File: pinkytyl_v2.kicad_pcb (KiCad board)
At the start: 2 copper layers, 132.2 x 106 mm, 58 parts, among them J1 STX-3501-3N, J2 Conn_01x02, J3 USB_B_Mini, J5 Conn_02x05_Odd_Even, K0 KEYSW, K10 KEYSW, K11 KEYSW, K12 KEYSW, K13 KEYSW, K14 KEYSW, K15 KEYSW, K20 KEYSW, K21 KEYSW, K22 KEYSW, K23 KEYSW, K24 KEYSW, K25 KEYSW, K30 KEYSW, K31 KEYSW, K32 KEYSW, K33 KEYSW, K34 KEYSW, K35 KEYSW, K40 KEYSW, K41 KEYSW, U1 ATmega32U4-MU, Y1 Crystal_GND24_Small

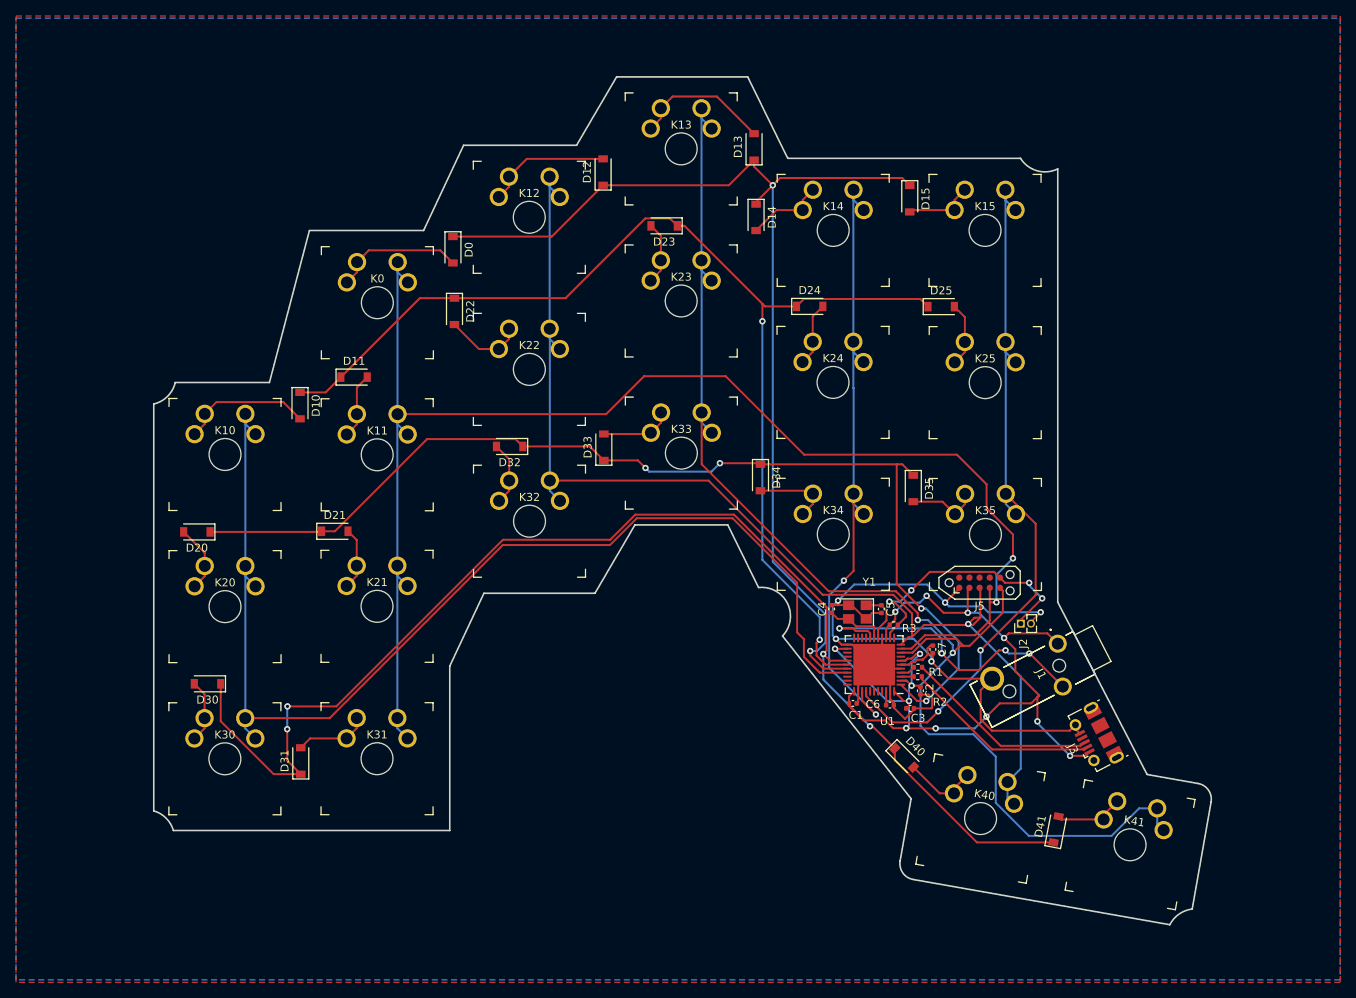
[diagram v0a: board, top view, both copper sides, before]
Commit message: In the middle of slim redesign
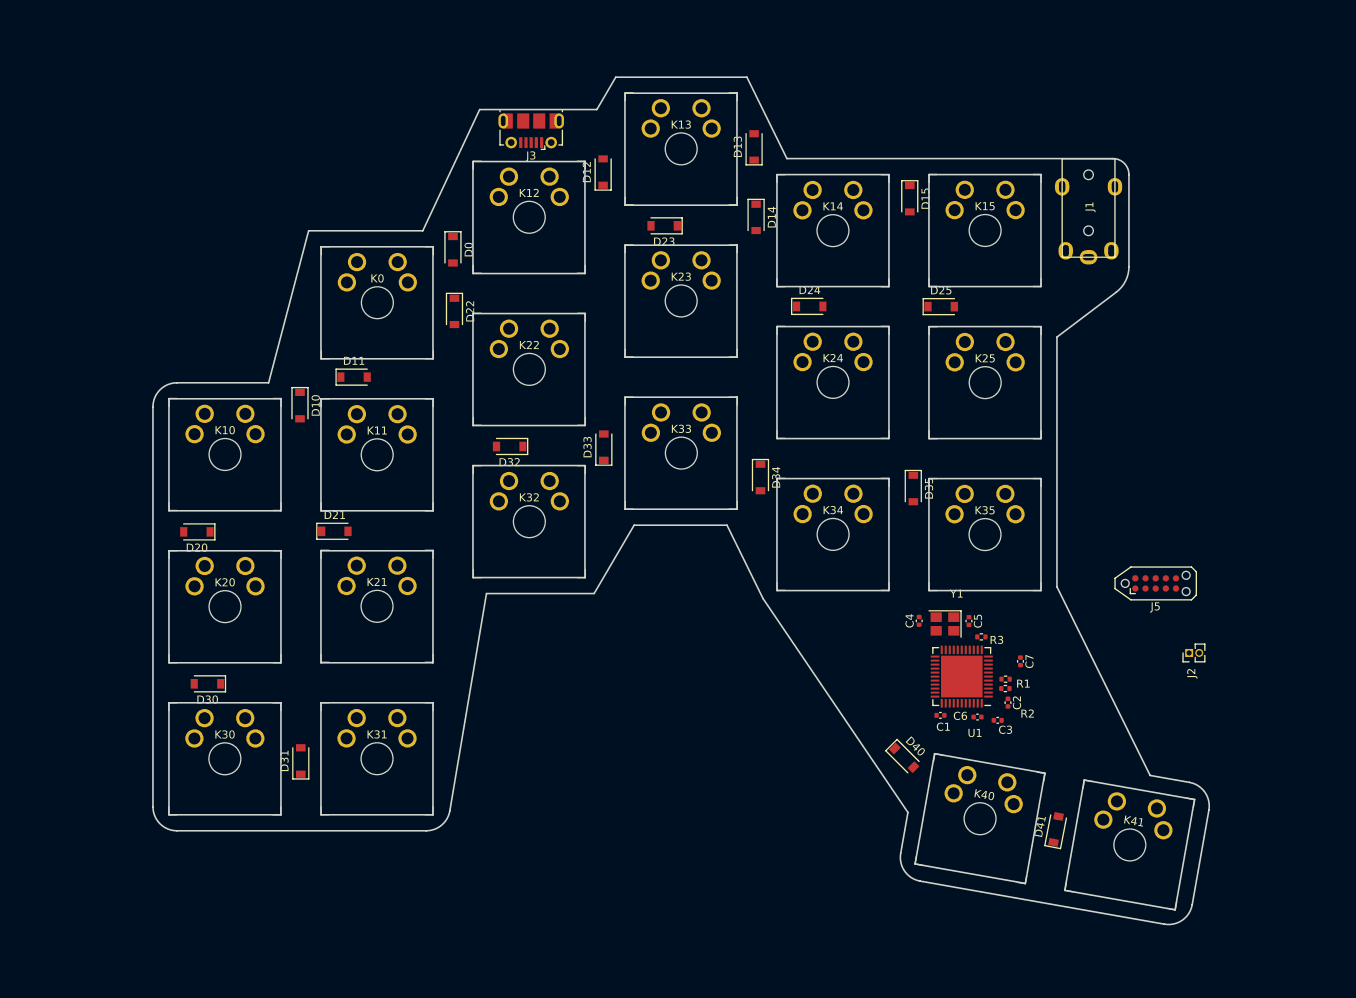
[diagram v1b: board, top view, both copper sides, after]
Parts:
- J1: value STX-3501-3N -> 50-00174; footprint STX-3501-3N:STX35013N -> misc:54-00174
- moved J3 103.5 mm to (117.8, 42.9), turned to 180 degrees
- moved J1 60.7 mm to (187.5, 46.4), turned to 270 degrees
- moved J5 22.0 mm to (195.9, 99.5)
- moved J2 21.4 mm to (200.1, 108.2)
- moved R1 11.1 mm to (177.2, 111.4)
- moved R2 11.1 mm to (177.1, 112.6)
- moved R3 11.1 mm to (174.1, 106.1)
- moved Y1 11.1 mm to (169.6, 104.5)
- moved C1 11.1 mm to (169.0, 116.0)
- moved C7 11.1 mm to (179.0, 109.2)
- moved C2 11.1 mm to (177.4, 114.4)
- moved C3 11.1 mm to (176.2, 116.6)
- moved C4 11.1 mm to (166.3, 104.1)
- moved C5 11.1 mm to (172.6, 104.2)
- moved C6 11.1 mm to (173.6, 116.2)
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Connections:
- J1 pad 2: GND -> serial
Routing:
- net MOSI: track 185.0 -> 0.00 mm, vias 2 -> 0
- net c3: track 171.3 -> 0.00 mm, vias 2 -> 0
- net r0: track 159.4 -> 0.00 mm, vias 4 -> 0
- net c0: track 145.8 -> 0.00 mm
- net MISO: track 144.7 -> 0.00 mm, vias 1 -> 0
- net r2: track 144.3 -> 0.00 mm, vias 2 -> 0
- net r3: track 135.0 -> 0.00 mm, vias 2 -> 0
- net r1: track 134.3 -> 0.00 mm, vias 4 -> 0
- net GND: track 122.4 -> 0.00 mm, vias 5 -> 0
- net VCC: track 113.2 -> 0.00 mm, vias 13 -> 0
- net c5: track 92.6 -> 0.00 mm, vias 2 -> 0
- net c4: track 82.1 -> 0.00 mm, vias 2 -> 0
- net serial: track 38.8 -> 0.00 mm, vias 4 -> 0
- net reset: track 33.0 -> 0.00 mm, vias 4 -> 0
- net d-: track 24.7 -> 0.00 mm
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- removed copper zone on B.Cu, net GND
- removed copper zone on F.Cu, net GND
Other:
- board size 132.2 x 106 mm -> 132 x 105.9 mm
